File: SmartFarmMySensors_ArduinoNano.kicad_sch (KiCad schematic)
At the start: 19 parts, among them J1 Conn_01x03, J2 Conn_01x03, J3 Conn_01x03, J4 Conn_01x03, J5 Screw_Terminal_01x03, J6 Screw_Terminal_01x03, J7 Power 5V, K1 Relay_SPDT, K2 Relay_SPDT, Q1 AO3400A, Q2 AO3400A, U1 NRF24L01_Breakout

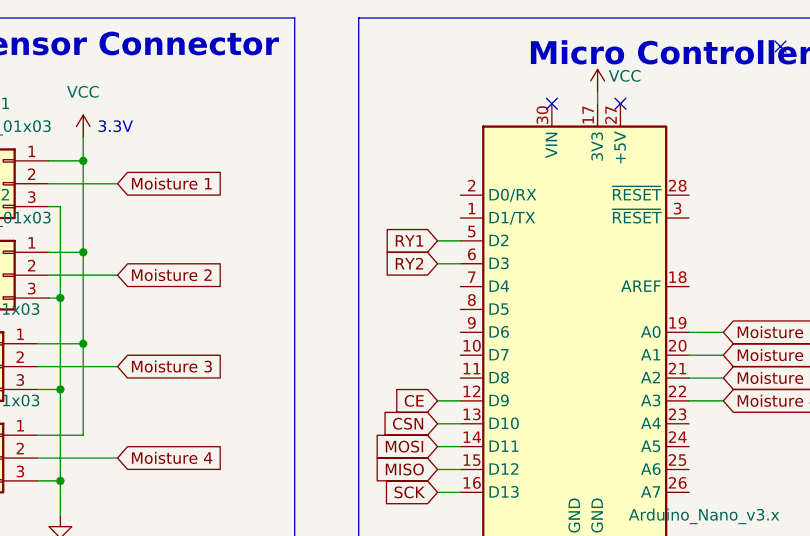
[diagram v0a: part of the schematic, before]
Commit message: ready to order
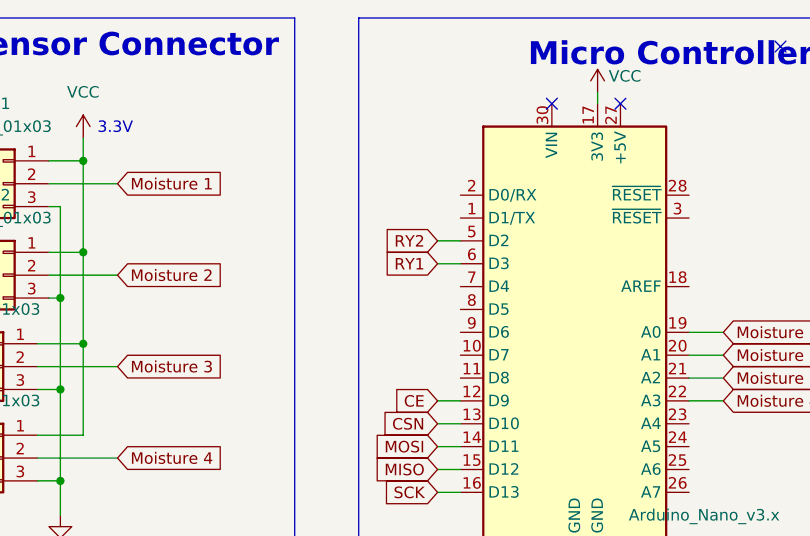
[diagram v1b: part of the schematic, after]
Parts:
- D1, D2: footprint (none) -> Diode_SMD:D_SMA
- J7: footprint TerminalBlock:TerminalBlock_Xinya_XY308-2.54-3P_1x03_P2.54mm_Horizontal -> TerminalBlock:TerminalBlock_Xinya_XY308-2.54-2P_1x02_P2.54mm_Horizontal
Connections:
- net RY1: now also A1.6 (D3); no longer A1.5 (D2)
- net RY2: now also A1.5 (D2); no longer A1.6 (D3)
